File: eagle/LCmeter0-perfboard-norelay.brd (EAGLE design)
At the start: 63.5 x 49.5 mm, 25 parts, among them IC1 PIC16F876A-X/SP, K2 DS2Y, Q1 20MHz, Q2 BC548, SW1 SPST, SW2 DPDT

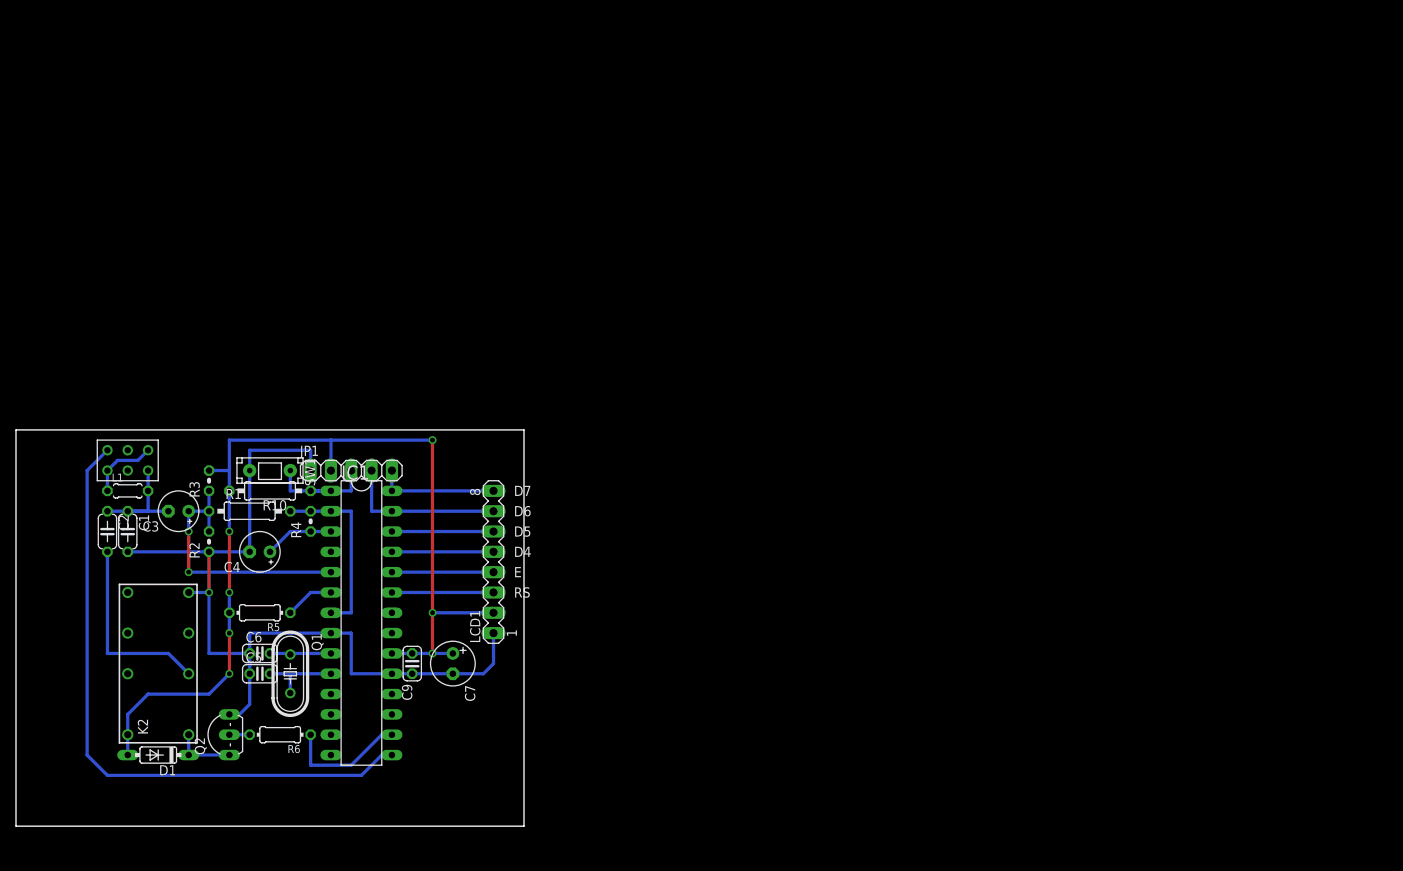
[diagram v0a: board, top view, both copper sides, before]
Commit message: ...
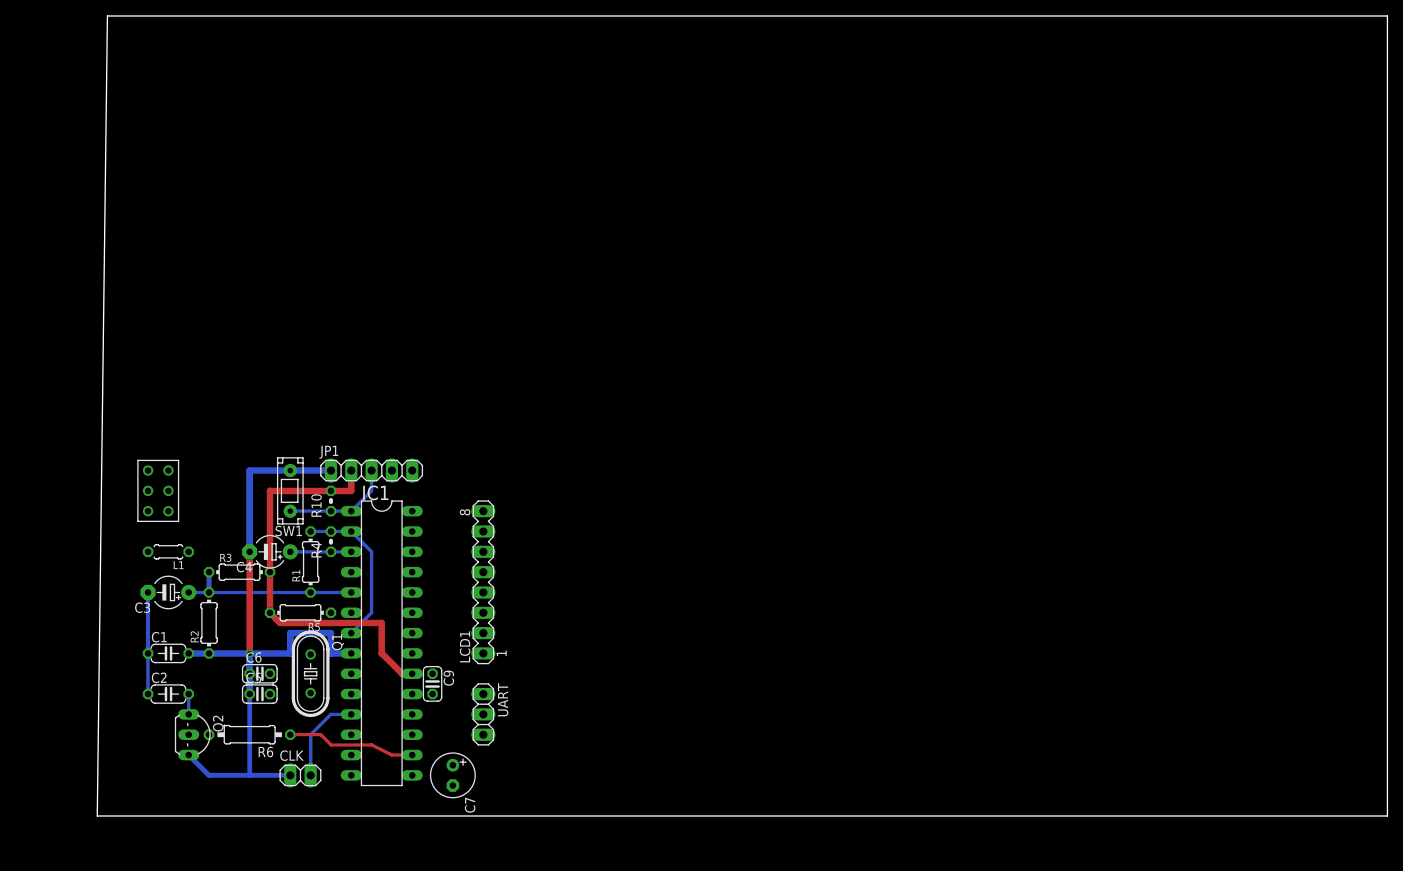
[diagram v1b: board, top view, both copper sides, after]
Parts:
- removed D1: 1N4148, diode:DO35-7
- removed K2: DS2Y, relay:DS2Y
- added CLK: (no value), pinhead:1X02
- added UART: (no value), pinhead:1X03
- C3, C4: device rcl:E2,5-5 -> rcl:E5-4
- L1: value 330u -> 860u
- R1: device rcl:0207/10 -> rcl:0204/7
- R10: device resistor:0207/10 -> resistor:0204V
- R2, R3: device resistor:0204V -> resistor:0204/7
- R6: device resistor:0204/7 -> resistor:0207/10
- moved C2 21.7 mm to (7.62, 15.2), turned to 0 degrees
- moved C1 16.1 mm to (7.62, 20.3), turned to 0 degrees
- moved C7 14.0 mm to (43.2, 5.08)
- moved R3 12.0 mm to (16.5, 30.5), turned to 0 degrees
- moved C3 10.2 mm to (7.62, 27.9)
- moved R2 10.2 mm to (12.7, 24.1)
- moved R1 9.92 mm to (25.4, 31.8), turned to 90 degrees
- moved L1 9.16 mm to (7.62, 33.0), turned to 180 degrees
- moved R10 7.73 mm to (27.9, 39.4), turned to 90 degrees
- moved SW1 7.62 mm to (24.1, 44.5), turned to 180 degrees
- moved SW2 5.39 mm to (6.35, 40.6), turned to 90 degrees
- moved R5 5.08 mm to (24.1, 25.4)
- moved R6 3.81 mm to (17.8, 10.2)
- moved R4 3.59 mm to (27.9, 34.3)
- moved C9 3.59 mm to (40.6, 16.5)
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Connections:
- net RC5 renamed CCAP
- removed net /RELAY: D1.C, K2.1, Q2.C
- new net N$1: CLK.2, IC1.11
- new net N$3: IC1.12
- new net RX: IC1.18, UART.2
- new net TX: IC1.17, UART.3
- net C2_CON: now also Q2.C; no longer K2.4
- net GND: now also CLK.1, UART.1; no longer K2.8
- net VCC: no longer D1.A, K2.16
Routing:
- net /LC: track 79.4 -> 0.00 mm
- net VCC: track 122.8 -> 51.1 mm, vias 7 -> 0
- net C2_CON: track 23.9 -> 2.54 mm
- net D6: track 20.3 -> 0.00 mm
- net D7: track 15.2 -> 0.00 mm
- net RS: track 12.7 -> 0.00 mm
- net E: track 12.7 -> 0.00 mm
- net D5: track 12.7 -> 0.00 mm
- net D4: track 12.7 -> 0.00 mm
- net N$1: track 0.00 -> 11.2 mm
- net GND: track 110.3 -> 100.1 mm
- net A3: track 33.0 -> 22.9 mm, vias 2 -> 0
- net OSC2: track 10.0 -> 0.00 mm
- net N$7: track 8.67 -> 0.00 mm
- net OSC1: track 7.75 -> 0.00 mm
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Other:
- board size 63.5 x 49.5 mm -> 161.3 x 100 mm
- board text removed: "D4"
- board text removed: "D5"
- board text removed: "D6"
- board text removed: "D7"
- board text removed: "E"
- board text removed: "RS"

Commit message: ...
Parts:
- IC1: device lc-meter:DIL28-3 -> mcu:DIL28-3
- SW1: device lc-meter:PB-5-1 -> mcu:PB-5-1
- SW2: device lc-meter:DPDT -> mcu:DPDT
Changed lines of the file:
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@@
 <element name="C9" library="rcl" package="C025-024X044" value="100nF" x="40.64" y="16.51" rot="R270"/>
 <element name="CLK" library="pinhead" package="1X02" value="" x="24.13" y="5.08"/>
-<element name="IC1" library="lc-meter" package="DIL28-3" value="PIC16F876A-X/SP" x="34.29" y="21.59" rot="R270"/>
+<element name="IC1" library="mcu" package="DIL28-3" value="PIC16F876A-X/SP" x="34.29" y="21.59" rot="R270"/>
 <element name="JP1" library="pinhead" package="1X05" value="" x="33.02" y="43.18"/>
 <element name="L1" library="rcl" package="0204/5" value="860u" x="7.62" y="33.02" rot="R180"/>
@@
 <element name="R5" library="resistor" package="0204/7" value="4.7kΩ" x="24.13" y="25.4" rot="R180"/>
 <element name="R6" library="resistor" package="0207/10" value="10kΩ" x="17.78" y="10.16" rot="R180"/>
-<element name="SW1" library="lc-meter" package="PB-5-1" value="SPST" x="24.13" y="44.45" rot="R180"/>
-<element name="SW2" library="lc-meter" package="DPDT" value="DPDT" x="6.35" y="40.64" rot="R90"/>
+<element name="SW1" library="mcu" package="PB-5-1" value="SPST" x="24.13" y="44.45" rot="R180"/>
+<element name="SW2" library="mcu" package="DPDT" value="DPDT" x="6.35" y="40.64" rot="R90"/>
 <element name="UART" library="pinhead" package="1X03" value="" x="46.99" y="12.7" rot="R270"/>
 </elements>

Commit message: ...
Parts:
- Q1: device crystal:HC49/S -> q:HC49/S
- Q2: device transistor-npn:TO92-EBC -> t:TO92-EBC
- R10, R4: device resistor:0204V -> r:0204V
- R2, R3, R5: device resistor:0204/7 -> r:0204/7
- R6: device resistor:0207/10 -> r:0207/10
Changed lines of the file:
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@@
 <attribute name="MF" value="" x="46.99" y="29.21" size="1.778" layer="27" rot="R90" display="off"/>
 </element>
-<element name="Q1" library="crystal" package="HC49/S" value="20MHz" x="25.4" y="17.78" rot="R270">
+<element name="Q1" library="q" package="HC49/S" value="20MHz" x="25.4" y="17.78" rot="R270">
 <attribute name="OC_NEWARK" value="unknown" x="25.4" y="17.78" size="1.778" layer="27" rot="R270" display="off"/>
 <attribute name="MPN" value="" x="25.4" y="17.78" size="1.778" layer="27" rot="R270" display="off"/>
@@
 <attribute name="MF" value="" x="25.4" y="17.78" size="1.778" layer="27" rot="R270" display="off"/>
 </element>
-<element name="Q2" library="transistor-npn" package="TO92-EBC" value="BC548" x="11.43" y="10.16" rot="R270"/>
+<element name="Q2" library="t" package="TO92-EBC" value="BC548" x="11.43" y="10.16" rot="R270"/>
 <element name="R1" library="rcl" package="0204/7" value="100kΩ" x="25.4" y="31.75" rot="R90"/>
-<element name="R10" library="resistor" package="0204V" value="4.7kΩ" x="27.94" y="39.37" rot="R90"/>
-<element name="R2" library="resistor" package="0204/7" value="100kΩ" x="12.7" y="24.13" rot="R90"/>
-<element name="R3" library="resistor" package="0204/7" value="100kΩ" x="16.51" y="30.48"/>
-<element name="R4" library="resistor" package="0204V" value="47kΩ" x="27.94" y="34.29" rot="R90"/>
-<element name="R5" library="resistor" package="0204/7" value="4.7kΩ" x="24.13" y="25.4" rot="R180"/>
-<element name="R6" library="resistor" package="0207/10" value="10kΩ" x="17.78" y="10.16" rot="R180"/>
+<element name="R10" library="r" package="0204V" value="4.7kΩ" x="27.94" y="39.37" rot="R90"/>
+<element name="R2" library="r" package="0204/7" value="100kΩ" x="12.7" y="24.13" rot="R90"/>
+<element name="R3" library="r" package="0204/7" value="100kΩ" x="16.51" y="30.48"/>
+<element name="R4" library="r" package="0204V" value="47kΩ" x="27.94" y="34.29" rot="R90"/>
+<element name="R5" library="r" package="0204/7" value="4.7kΩ" x="24.13" y="25.4" rot="R180"/>
+<element name="R6" library="r" package="0207/10" value="10kΩ" x="17.78" y="10.16" rot="R180"/>
 <element name="SW1" library="mcu" package="PB-5-1" value="SPST" x="24.13" y="44.45" rot="R180"/>
 <element name="SW2" library="mcu" package="DPDT" value="DPDT" x="6.35" y="40.64" rot="R90"/>
